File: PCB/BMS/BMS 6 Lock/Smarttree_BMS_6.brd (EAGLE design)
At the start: 90.9 x 58.3 mm, 79 parts

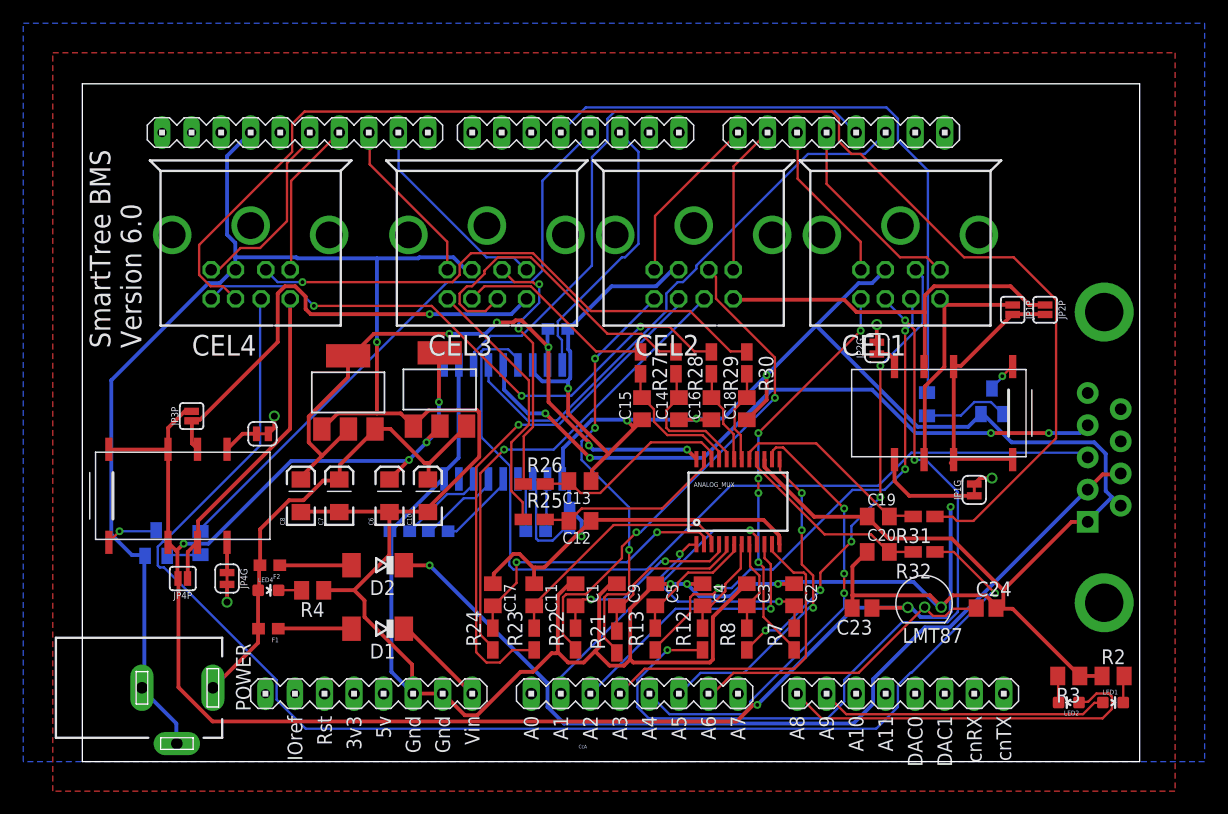
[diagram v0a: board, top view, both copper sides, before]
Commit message: gerbers
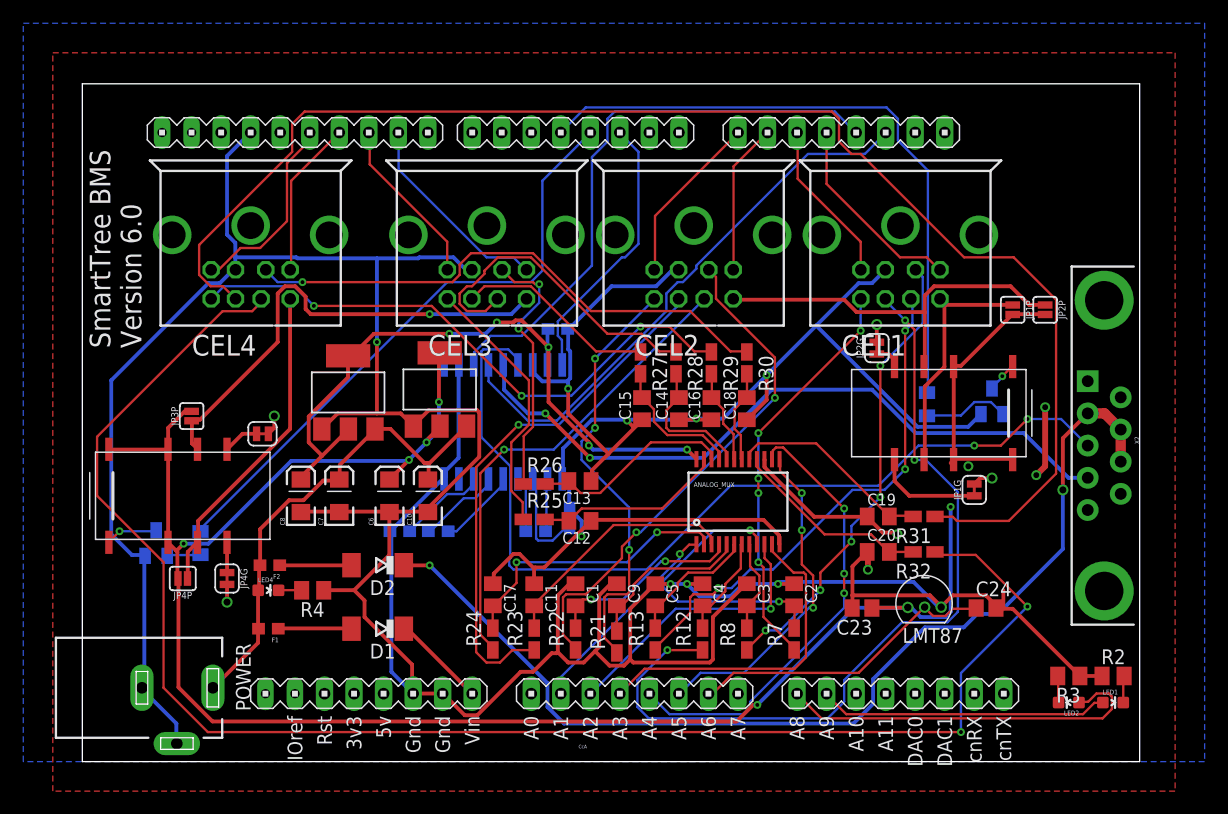
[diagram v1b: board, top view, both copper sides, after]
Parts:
- moved X2 1.02 mm to (87.9, 32.3), flipped to the top, turned to 270 degrees
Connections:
- net GND: now also X2.1, X2.6
- net SCRN_PWR: now also X2.7
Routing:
- net GND: track 505.8 -> 472.8 mm, vias 13 -> 17
- net VS4: track 118.0 -> 136.3 mm, vias 1 -> 2
- net SCRN_PWR: track 78.7 -> 89.7 mm, vias 1 -> 2
- net TX: track 77.8 -> 79.8 mm, vias 0 -> 2
- net CSI4: track 119.7 -> 121.5 mm
- net RX: track 59.0 -> 60.3 mm, vias 4 -> 2
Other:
- board text removed: "----Layout ->make it nicer ->put analog MUX on the top layer ->make a debugging interface for sensor reading ->switch bypass with jumper -> DONE make sensor board connectors closer to the edge -> add back 5V top and GND bottom planes"
